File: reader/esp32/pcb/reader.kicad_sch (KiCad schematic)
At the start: 28 parts, among them J1 Conn_01x06, J2 Conn_01x02, J3 Conn_01x04, J4 Conn_01x02, Q1 MMBT3904, Q2 MMBT3904, U1 ESP32-WROOM-32U, U2 RF125-PS, U3 CH340C, U4 74LVC1T45, U5 AMS1117-3.3

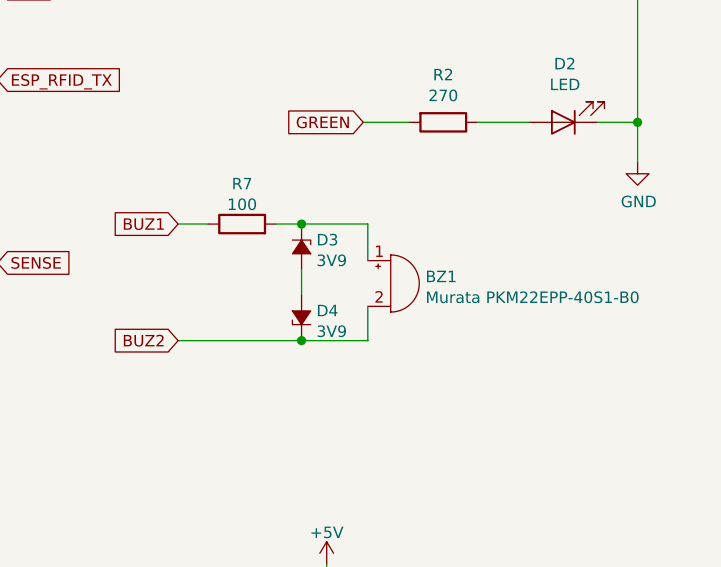
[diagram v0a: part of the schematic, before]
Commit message: Fix 3D models.
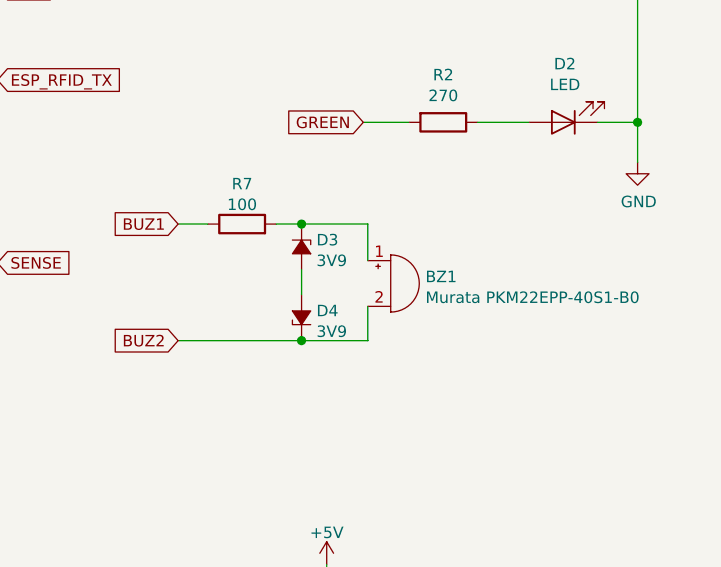
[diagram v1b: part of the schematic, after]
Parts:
- J4: footprint Connector_PinHeader_2.54mm:PinHeader_1x02_P2.54mm_Vertical -> Connector_JST:JST_XH_S02B-XH-A-1_1x02_P2.50mm_Horizontal
